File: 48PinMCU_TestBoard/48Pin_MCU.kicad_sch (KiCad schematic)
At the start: 32 parts, among them IC1 74LVC1G157GW,125, J5 SWD, SW1 Reset, SW2 SW_SPDT, U1 STM32G431CBT6, Y1 Crystal

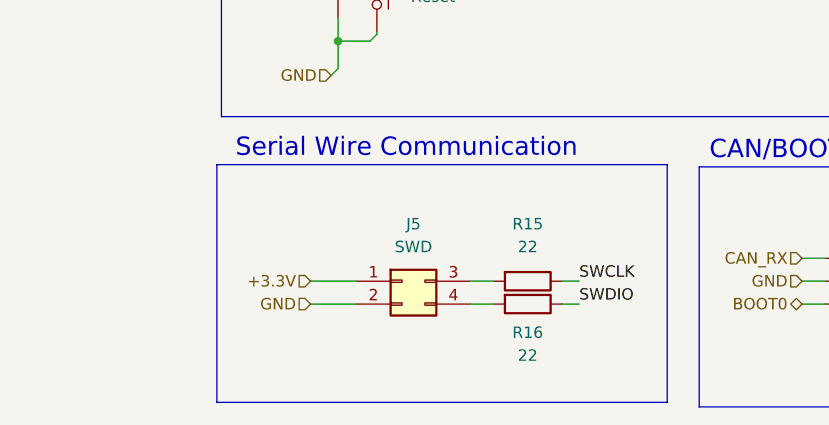
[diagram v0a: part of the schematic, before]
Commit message: layout tweaks
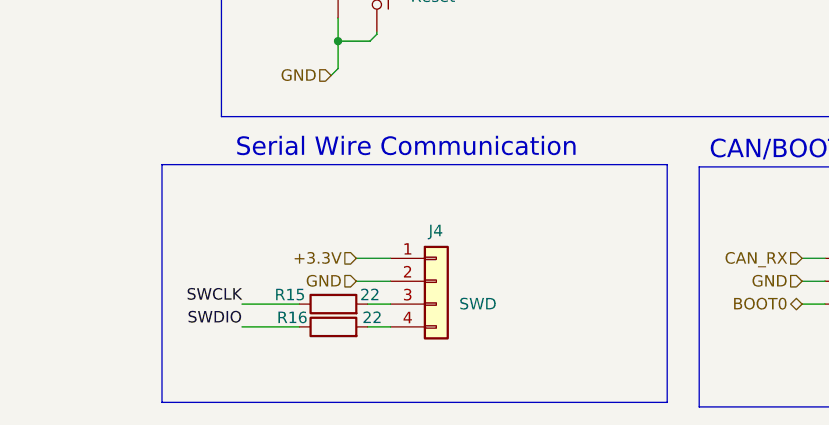
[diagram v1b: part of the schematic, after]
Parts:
- removed J5: SWD, UTSVT_Connectors:Molex_Nano-Fit_105309-xx04_1x04_P2.50mm_Vertical, symbol 100PinMCU:SWD_Header_02x02
- added J4: SWD, Connector_PinHeader_2.54mm:PinHeader_1x04_P2.54mm_Vertical, symbol Connector_Generic:Conn_01x04
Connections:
- net +3.3V: now also J4.1 (Pin_1)
- net GND: now also J4.2 (Pin_2)
- net at R15.2: now also J4.3 (Pin_3)
- net at R16.2: now also J4.4 (Pin_4)
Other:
- moved on the sheet: R15, R16
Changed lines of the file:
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@@
 	)
 	(rectangle
-		(start 164.846 136.906)
+		(start 158.75 136.906)
 		(end 214.884 163.322)
 		(stroke
@@
 	(wire
 		(pts
-			(xy 203.2 152.4) (xy 205.105 152.4)
+			(xy 173.99 154.94) (xy 167.64 154.94)
 		)
 		(stroke
@@
 	(wire
 		(pts
-			(xy 175.26 152.4) (xy 180.34 152.4)
+			(xy 180.34 149.86) (xy 184.15 149.86)
 		)
 		(stroke
@@
 	(wire
 		(pts
-			(xy 193.04 152.4) (xy 195.58 152.4)
+			(xy 184.15 154.94) (xy 181.61 154.94)
 		)
 		(stroke
@@
 	(wire
 		(pts
-			(xy 203.2 149.86) (xy 205.105 149.86)
+			(xy 173.99 152.4) (xy 167.64 152.4)
 		)
 		(stroke
@@
 	(wire
 		(pts
-			(xy 193.04 149.86) (xy 195.58 149.86)
+			(xy 184.15 152.4) (xy 181.61 152.4)
 		)
 		(stroke
@@
 	(wire
 		(pts
-			(xy 175.26 149.86) (xy 180.34 149.86)
+			(xy 180.34 147.32) (xy 184.15 147.32)
 		)
 		(stroke
@@
 	)
 	(label "SWCLK"
-		(at 205.105 149.86 0)
+		(at 167.64 152.4 180)
 		(effects
 			(font
 				(size 1.27 1.27)
 			)
-			(justify left bottom)
+			(justify right bottom)
 		)
 	)
@@
 	)
 	(label "SWDIO"
-		(at 205.105 152.4 0)
+		(at 167.64 154.94 180)
 		(effects
 			(font
 				(size 1.27 1.27)
 			)
-			(justify left bottom)
+			(justify right bottom)
 		)
 	)
@@
 	(hierarchical_label "GND"
 		(shape input)
-		(at 175.26 152.4 180)
+		(at 180.34 149.86 180)
 		(effects
 			(font
@@
 	(hierarchical_label "+3.3V"
 		(shape input)
-		(at 175.26 149.86 180)
+		(at 180.34 147.32 180)
 		(effects
 			(font
@@
 	)
 	(symbol
+		(lib_id "Connector_Generic:Conn_01x04")
+		(at 189.23 149.86 0)
+		(unit 1)
+		(exclude_from_sim no)
+		(in_bom yes)
+		(on_board yes)
+		(dnp no)
+		(property "Reference" "J4"
+			(at 189.992 144.272 0)
+			(effects
+				(font
+					(size 1.27 1.27)
+				)
+				(justify right)
+			)
+		)
+		(property "Value" "SWD"
+			(at 191.77 152.3999 0)
+			(effects
+				(font
+					(size 1.27 1.27)
+				)
+				(justify left)
+			)
+		)
+		(property "Footprint" "Connector_PinHeader_2.54mm:PinHeader_1x04_P2.54mm_Vertical"
+			(at 189.23 149.86 0)
+			(effects
+				(font
+					(size 1.27 1.27)
+				)
+				(hide yes)
+			)
+		)
+		(property "Datasheet" "~"
+			(at 189.23 149.86 0)
+			(effects
+				(font
+					(size 1.27 1.27)
+				)
+				(hide yes)
+			)
+		)
+		(property "Description" "Generic connector, single row, 01x04, script generated (kicad-library-utils/schlib/autogen/connector/)"
+			(at 189.23 149.86 0)
+			(effects
+				(font
+					(size 1.27 1.27)
+				)
+				(hide yes)
+			)
+		)
+		(pin "2"
+		)
+		(pin "1"
+		)
+		(pin "4"
+		)
+		(pin "3"
+		)
+		(instances
+			(project ""
+				(path "/9cc459e0-f86d-41bb-8426-cce80d92e44c/f864dc39-a41c-4593-ac23-dc35fa5d1c83"
+					(reference "J4")
+					(unit 1)
+				)
+			)
+		)
+	)
+	(symbol
 		(lib_id "Device:R")
-		(at 199.39 149.86 270)
+		(at 177.8 152.4 90)
 		(unit 1)
 		(exclude_from_sim no)
@@
 		(on_board yes)
 		(dnp no)
-		(fields_autoplaced yes)
 		(property "Reference" "R15"
-			(at 199.39 143.51 90)
+			(at 172.974 151.384 90)
 			(effects
 				(font
@@
 		)
 		(property "Value" "22"
-			(at 199.39 146.05 90)
+			(at 181.864 151.384 90)
 			(effects
 				(font
@@
 		)
 		(property "Footprint" "Resistor_SMD:R_0603_1608Metric_Pad0.98x0.95mm_HandSolder"
-			(at 199.39 148.082 90)
+			(at 177.8 154.178 90)
 			(effects
 				(font
@@
 		)
 		(property "Datasheet" "~"
-			(at 199.39 149.86 0)
+			(at 177.8 152.4 0)
 			(effects
 				(font
@@
 		)
 		(property "Description" "Resistor"
-			(at 199.39 149.86 0)
+			(at 177.8 152.4 0)
 			(effects
 				(font
@@
 		)
 		(property "LCSC P/N" "C25804"
-			(at 199.39 149.86 90)
+			(at 177.8 152.4 90)
 			(effects
 				(font
@@
 		)
 		(property "P/N" "FRC0603F22R0TS"
-			(at 199.39 149.86 90)
+			(at 177.8 152.4 90)
 			(effects
 				(font
@@
 	(symbol
 		(lib_id "Device:R")
-		(at 199.39 152.4 270)
+		(at 177.8 154.94 90)
 		(unit 1)
 		(exclude_from_sim no)
@@
 		(dnp no)
 		(property "Reference" "R16"
-			(at 199.39 155.575 90)
+			(at 173.228 153.924 90)
 			(effects
 				(font
@@
 		)
 		(property "Value" "22"
-			(at 199.39 158.115 90)
+			(at 182.118 153.924 90)
 			(effects
 				(font
@@
 		)
 		(property "Footprint" "Resistor_SMD:R_0603_1608Metric_Pad0.98x0.95mm_HandSolder"
-			(at 199.39 150.622 90)
+			(at 177.8 156.718 90)
 			(effects
 				(font
@@
 		)
 		(property "Datasheet" "~"
-			(at 199.39 152.4 0)
+			(at 177.8 154.94 0)
 			(effects
 				(font
@@
 		)
 		(property "Description" "Resistor"
-			(at 199.39 152.4 0)
+			(at 177.8 154.94 0)
 			(effects
 				(font
@@
 		)
 		(property "LCSC P/N" "C25804"
-			(at 199.39 152.4 90)
+			(at 177.8 154.94 90)
 			(effects
 				(font
@@
 		)
 		(property "P/N" "FRC0603F22R0TS"
-			(at 199.39 152.4 90)
+			(at 177.8 154.94 90)
 			(effects
 				(font
@@
 					(unit 1)
 				)
-			)
-		)
-	)
-	(symbol
-		(lib_id "100PinMCU:SWD_Header_02x02")
-		(at 185.42 149.86 0)
-		(unit 1)
-		(exclude_from_sim no)
-		(in_bom yes)
-		(on_board yes)
-		(dnp no)
-		(fields_autoplaced yes)
-		(property "Reference" "J5"
-			(at 186.69 143.51 0)
-			(effects
-				(font
-					(size 1.27 1.27)
-				)
-			)
-		)
-		(property "Value" "SWD"
-			(at 186.69 146.05 0)
-			(effects
-				(font
-					(size 1.27 1.27)
-				)
-			)
-		)
-		(property "Footprint" "UTSVT_Connectors:Molex_Nano-Fit_105309-xx04_1x04_P2.50mm_Vertical"
-			(at 185.42 149.86 0)
-			(effects
-				(font
-					(size 1.27 1.27)
-				)
-				(hide yes)
-			)
-		)
-		(property "Datasheet" "kicad-embed://Conn_02x02_Odd_Even.pdf"
-			(at 185.42 149.86 0)
-			(effects
-				(font
-					(size 1.27 1.27)
-				)
-				(hide yes)
-			)
-		)
-		(property "Description" "Generic connector, double row, 02x02, odd/even pin numbering scheme (row 1 odd numbers, row 2 even numbers), script generated (kicad-library-utils/schlib/autogen/connector/)"
-			(at 185.42 149.86 0)
-			(effects
-				(font
-					(size 1.27 1.27)
-				)
-				(hide yes)
-			)
-		)
-		(property "P/N" "0878320406"
-			(at 185.42 149.86 0)
-			(effects
-				(font
-					(size 1.27 1.27)
-				)
-				(hide yes)
-			)
-		)
-		(property "LCSC P/N" "C17492485"
-			(at 185.42 149.86 0)
-			(effects
-				(font
-					(size 1.27 1.27)
-				)
-				(hide yes)
-			)
-		)
-		(pin "2"
-		)
-		(pin "1"
-		)
-		(pin "4"
-		)
-		(pin "3"
-		)
-		(instances
-			(project ""
-				(path "/9cc459e0-f86d-41bb-8426-cce80d92e44c/f864dc39-a41c-4593-ac23-dc35fa5d1c83"
-					(reference "J5")
-					(unit 1)
-				)
-			)
-			(project "48PinMCU"
-				(path "/b973e36d-c926-4cad-b0c3-dce51444ffeb"
-					(reference "J1")
-					(unit 1)
-				)

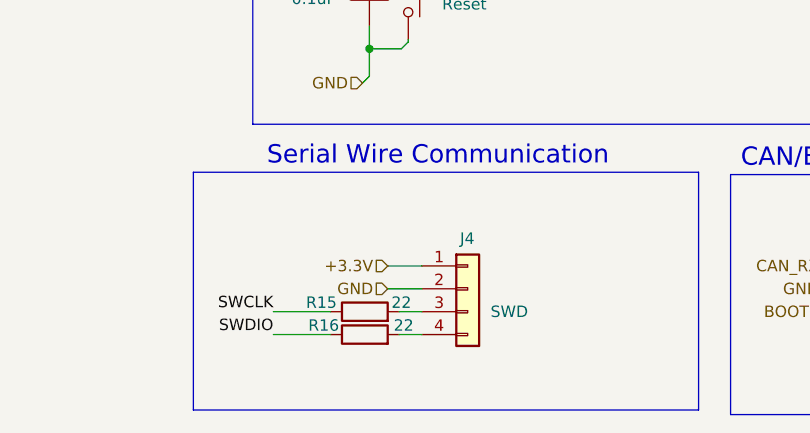
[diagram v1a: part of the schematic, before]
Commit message: temp
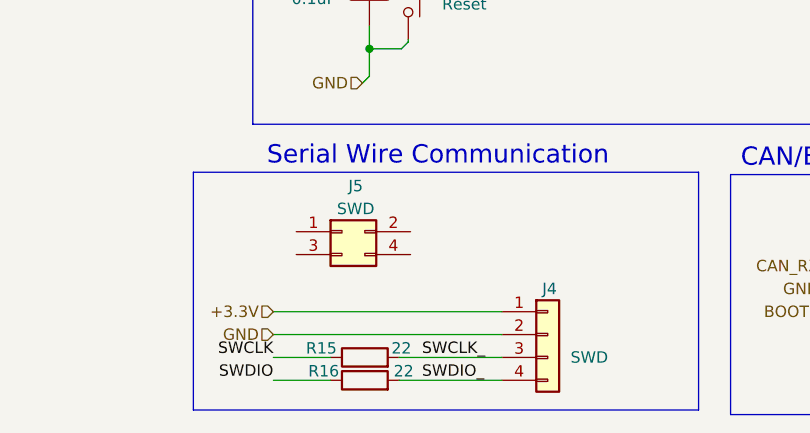
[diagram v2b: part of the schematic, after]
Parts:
- added J5: SWD, symbol Connector_Generic:Conn_02x02_Odd_Even
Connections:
- net SWCLK_: now reaches J4.3 (Pin_3), R15.2
- net SWDIO_: now reaches J4.4 (Pin_4), R16.2
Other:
- moved on the sheet: J4, R15, R16
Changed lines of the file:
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@@
 	(wire
 		(pts
-			(xy 173.99 154.94) (xy 167.64 154.94)
+			(xy 173.99 160.02) (xy 167.64 160.02)
 		)
 		(stroke
@@
 	(wire
 		(pts
-			(xy 180.34 149.86) (xy 184.15 149.86)
+			(xy 167.64 154.94) (xy 193.04 154.94)
 		)
 		(stroke
@@
 	(wire
 		(pts
-			(xy 184.15 154.94) (xy 181.61 154.94)
+			(xy 181.61 160.02) (xy 193.04 160.02)
 		)
 		(stroke
@@
 	(wire
 		(pts
-			(xy 173.99 152.4) (xy 167.64 152.4)
+			(xy 173.99 157.48) (xy 167.64 157.48)
 		)
 		(stroke
@@
 	(wire
 		(pts
-			(xy 184.15 152.4) (xy 181.61 152.4)
+			(xy 181.61 157.48) (xy 193.04 157.48)
 		)
 		(stroke
@@
 	(wire
 		(pts
-			(xy 180.34 147.32) (xy 184.15 147.32)
+			(xy 167.64 152.4) (xy 193.04 152.4)
 		)
 		(stroke
@@
 	)
 	(label "SWCLK"
-		(at 167.64 152.4 180)
+		(at 167.64 157.48 180)
 		(effects
 			(font
@@
 		)
 	)
+	(label "SWDIO_"
+		(at 184.15 160.02 0)
+		(effects
+			(font
+				(size 1.27 1.27)
+			)
+			(justify left bottom)
+		)
+	)
 	(label "CAN_RX{slash}BOOT0"
 		(at 271.78 152.4 180)
@@
 	)
 	(label "SWDIO"
-		(at 167.64 154.94 180)
+		(at 167.64 160.02 180)
 		(effects
 			(font
@@
 		)
 	)
+	(label "SWCLK_"
+		(at 184.15 157.48 0)
+		(effects
+			(font
+				(size 1.27 1.27)
+			)
+			(justify left bottom)
+		)
+	)
 	(label "SWDIO"
 		(at 24.13 71.12 0)
@@
 	(hierarchical_label "GND"
 		(shape input)
-		(at 180.34 149.86 180)
+		(at 167.64 154.94 180)
 		(effects
 			(font
@@
 	(hierarchical_label "+3.3V"
 		(shape input)
-		(at 180.34 147.32 180)
+		(at 167.64 152.4 180)
 		(effects
 			(font
@@
 	)
 	(symbol
+		(lib_id "Connector_Generic:Conn_02x02_Odd_Even")
+		(at 175.26 143.51 0)
+		(unit 1)
+		(exclude_from_sim no)
+		(in_bom yes)
+		(on_board yes)
+		(dnp no)
+		(property "Reference" "J5"
+			(at 176.784 138.43 0)
+			(effects
+				(font
+					(size 1.27 1.27)
+				)
+			)
+		)
+		(property "Value" "SWD"
+			(at 176.784 140.97 0)
+			(effects
+				(font
+					(size 1.27 1.27)
+				)
+			)
+		)
+		(property "Footprint" ""
+			(at 175.26 143.51 0)
+			(effects
+				(font
+					(size 1.27 1.27)
+				)
+				(hide yes)
+			)
+		)
+		(property "Datasheet" "~"
+			(at 175.26 143.51 0)
+			(effects
+				(font
+					(size 1.27 1.27)
+				)
+				(hide yes)
+			)
+		)
+		(property "Description" "Generic connector, double row, 02x02, odd/even pin numbering scheme (row 1 odd numbers, row 2 even numbers), script generated (kicad-library-utils/schlib/autogen/connector/)"
+			(at 175.26 143.51 0)
+			(effects
+				(font
+					(size 1.27 1.27)
+				)
+				(hide yes)
+			)
+		)
+		(pin "3"
+		)
+		(pin "1"
+		)
+		(pin "2"
+		)
+		(pin "4"
+		)
+		(instances
+			(project ""
+				(path "/9cc459e0-f86d-41bb-8426-cce80d92e44c/f864dc39-a41c-4593-ac23-dc35fa5d1c83"
+					(reference "J5")
+					(unit 1)
+				)
+			)
+		)
+	)
+	(symbol
 		(lib_id "Connector_Generic:Conn_01x04")
-		(at 189.23 149.86 0)
+		(at 198.12 154.94 0)
 		(unit 1)
 		(exclude_from_sim no)
@@
 		(dnp no)
 		(property "Reference" "J4"
-			(at 189.992 144.272 0)
+			(at 199.136 149.86 0)
 			(effects
 				(font
@@
 		)
 		(property "Value" "SWD"
-			(at 191.77 152.3999 0)
+			(at 200.66 157.4799 0)
 			(effects
 				(font
@@
 		)
 		(property "Footprint" "Connector_PinHeader_2.54mm:PinHeader_1x04_P2.54mm_Vertical"
-			(at 189.23 149.86 0)
+			(at 198.12 154.94 0)
 			(effects
 				(font
@@
 		)
 		(property "Datasheet" "~"
-			(at 189.23 149.86 0)
+			(at 198.12 154.94 0)
 			(effects
 				(font
@@
 		)
 		(property "Description" "Generic connector, single row, 01x04, script generated (kicad-library-utils/schlib/autogen/connector/)"
-			(at 189.23 149.86 0)
+			(at 198.12 154.94 0)
 			(effects
 				(font
@@
 	(symbol
 		(lib_id "Device:R")
-		(at 177.8 152.4 90)
+		(at 177.8 157.48 90)
 		(unit 1)
 		(exclude_from_sim no)
@@
 		(dnp no)
 		(property "Reference" "R15"
-			(at 172.974 151.384 90)
+			(at 172.974 156.464 90)
 			(effects
 				(font
@@
 		)
 		(property "Value" "22"
-			(at 181.864 151.384 90)
+			(at 181.864 156.464 90)
 			(effects
 				(font
@@
 		)
 		(property "Footprint" "Resistor_SMD:R_0603_1608Metric_Pad0.98x0.95mm_HandSolder"
-			(at 177.8 154.178 90)
+			(at 177.8 159.258 90)
 			(effects
 				(font
@@
 		)
 		(property "Datasheet" "~"
-			(at 177.8 152.4 0)
+			(at 177.8 157.48 0)
 			(effects
 				(font
@@
 		)
 		(property "Description" "Resistor"
-			(at 177.8 152.4 0)
+			(at 177.8 157.48 0)
 			(effects
 				(font
@@
 		)
 		(property "LCSC P/N" "C25804"
-			(at 177.8 152.4 90)
+			(at 177.8 157.48 90)
 			(effects
 				(font
@@
 		)
 		(property "P/N" "FRC0603F22R0TS"
-			(at 177.8 152.4 90)
+			(at 177.8 157.48 90)
 			(effects
 				(font
@@
 	(symbol
 		(lib_id "Device:R")
-		(at 177.8 154.94 90)
+		(at 177.8 160.02 90)
 		(unit 1)
 		(exclude_from_sim no)
@@
 		(dnp no)
 		(property "Reference" "R16"
-			(at 173.228 153.924 90)
+			(at 173.228 159.004 90)
 			(effects
 				(font
@@
 		)
 		(property "Value" "22"
-			(at 182.118 153.924 90)
+			(at 182.118 159.004 90)
 			(effects
 				(font
@@
 		)
 		(property "Footprint" "Resistor_SMD:R_0603_1608Metric_Pad0.98x0.95mm_HandSolder"
-			(at 177.8 156.718 90)
+			(at 177.8 161.798 90)
 			(effects
 				(font
@@
 		)
 		(property "Datasheet" "~"
-			(at 177.8 154.94 0)
+			(at 177.8 160.02 0)
 			(effects
 				(font
@@
 		)
 		(property "Description" "Resistor"
-			(at 177.8 154.94 0)
+			(at 177.8 160.02 0)
 			(effects
 				(font
@@
 		)
 		(property "LCSC P/N" "C25804"
-			(at 177.8 154.94 90)
+			(at 177.8 160.02 90)
 			(effects
 				(font
@@
 		)
 		(property "P/N" "FRC0603F22R0TS"
-			(at 177.8 154.94 90)
+			(at 177.8 160.02 90)
 			(effects
 				(font
